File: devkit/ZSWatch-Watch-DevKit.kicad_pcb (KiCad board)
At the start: 4 copper layers, 100 x 70 mm, 130 parts, among them IC401 nPM1300-QEXX, IC501 APDS-9306-065, IC502 BMI270, IC503 LIS2MDLTR, IC504 BMP581, IC505 DRV2603RUNT, IC506 PCA9306JK, IC507 RV-8263-C8, IC601 FAN5622SX, IC602 USBLC6-2P6, IC603 MX25U51245GZ4I00, IC604 NTS0104GU12, M601 NORA-B106, Q401 PMZ550UNEYL, Q402 PMZ550UNEYL, Q403 PMZ550UNEYL, Q404 PMZB320UPEYL, X401 Battery, X402 Battery, X403 Power, X404 VSYS, X501 Current, X502 I2S, X503 Current, X504 I2C, X505 Current, X506 Current, X507 Current, X508 Current, X509 Motor, X510 Current, X601 DEBUG, X602 Current, X603 Device, X604 UART, X605 GPIO, X606 Current, X607 IO Current, X608 Display, X609 Current, X610 LED Current

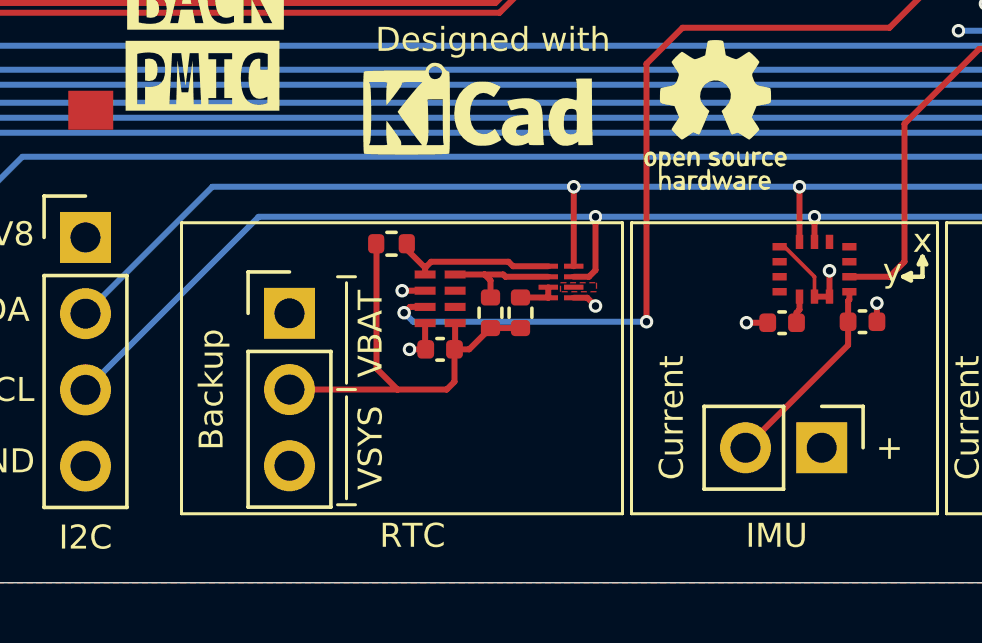
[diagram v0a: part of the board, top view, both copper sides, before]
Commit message: Revert "Feature: Issue #186"
This reverts commit 73512b60dac517a3d61ff56758c38d705b52f64d.
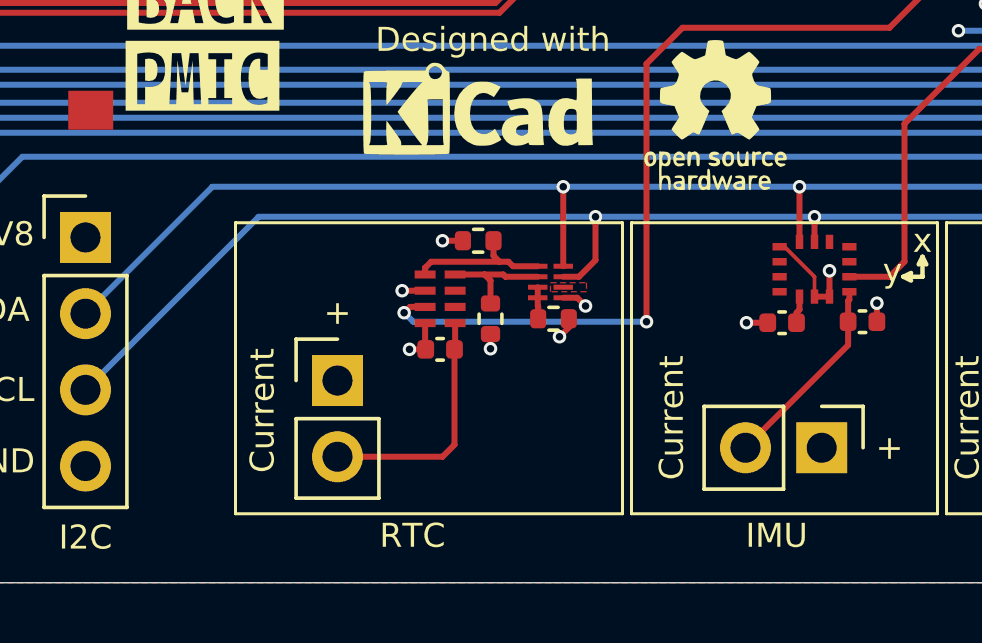
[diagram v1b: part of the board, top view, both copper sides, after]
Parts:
- X510: footprint Connector_PinHeader_2.54mm:PinHeader_1x03_P2.54mm_Vertical -> Connector_PinHeader_2.54mm:PinHeader_1x02_P2.54mm_Vertical
- moved R505 2.89 mm to (207.9, 172.6)
- moved X510 2.75 mm to (203.2, 177.3)
- moved R503 1.12 mm to (210.4, 175.2), turned to 0 degrees
- moved IC506 0.35 mm to (210.3, 174.0)
- moved R504 0.20 mm to (208.3, 175.2)
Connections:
- R503 pad 1: Net-(IC507-V_{DD}) -> Net-(IC506-EN)
- R503 pad 2: Net-(IC506-EN) -> /Project Architecture/Peripherals/VBAT
- R504 pad 2: Net-(IC507-V_{DD}) -> /Project Architecture/Peripherals/VBAT
- R505 pad 2: Net-(IC507-V_{DD}) -> /Project Architecture/Peripherals/VBAT
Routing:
- net /Project Architecture/Power Management/VSYS: track 274.0 -> 224.2 mm
- net Net-(IC507-V_{DD}): track 15.2 -> 8.13 mm
- net /Project Architecture/Peripherals/VBAT: track 22.1 -> 24.0 mm, vias 2 -> 5
- net Net-(IC506-SDA_{2}): track 5.53 -> 4.91 mm
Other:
- board text removed: "Backup"
- board text removed: "VBAT"
